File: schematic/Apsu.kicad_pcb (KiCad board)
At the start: 2 copper layers, 80 x 80 mm, 58 parts, among them J1 Conn_02x03_Odd_Even, J12 Conn_01x03, J13 Conn_01x02, J14 Conn_01x03_Female, J15 Conn_01x03, J16 Conn_01x03, J17 Conn_01x03, J18 Conn_01x02_Male, J19 Conn_01x02, J2 Conn_02x05_Odd_Even, J3 Conn_02x05_Odd_Even, J4 Conn_01x02, J5 Conn_01x02, J6 Conn_01x02, J7 Conn_01x02, J8 Conn_01x05, J9 Conn_01x08_Male, SW1 SW_DIP_x01, U1 ESP32-WROOM-32, U2 LM2595S-3.3, U3 PCA9685PW, U4 MAX11613, U5 MAX485E

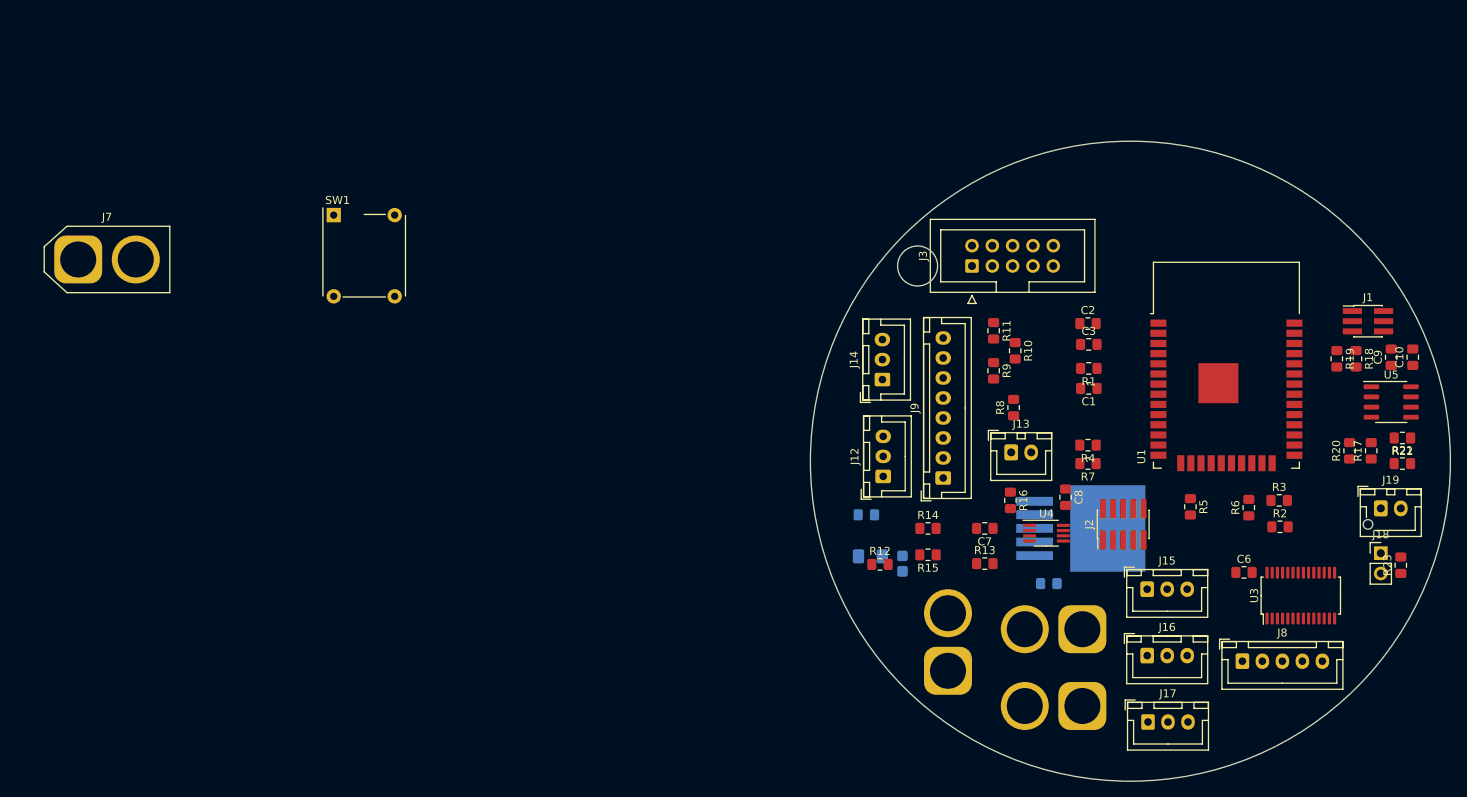
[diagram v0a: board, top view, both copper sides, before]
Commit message: new pcb design
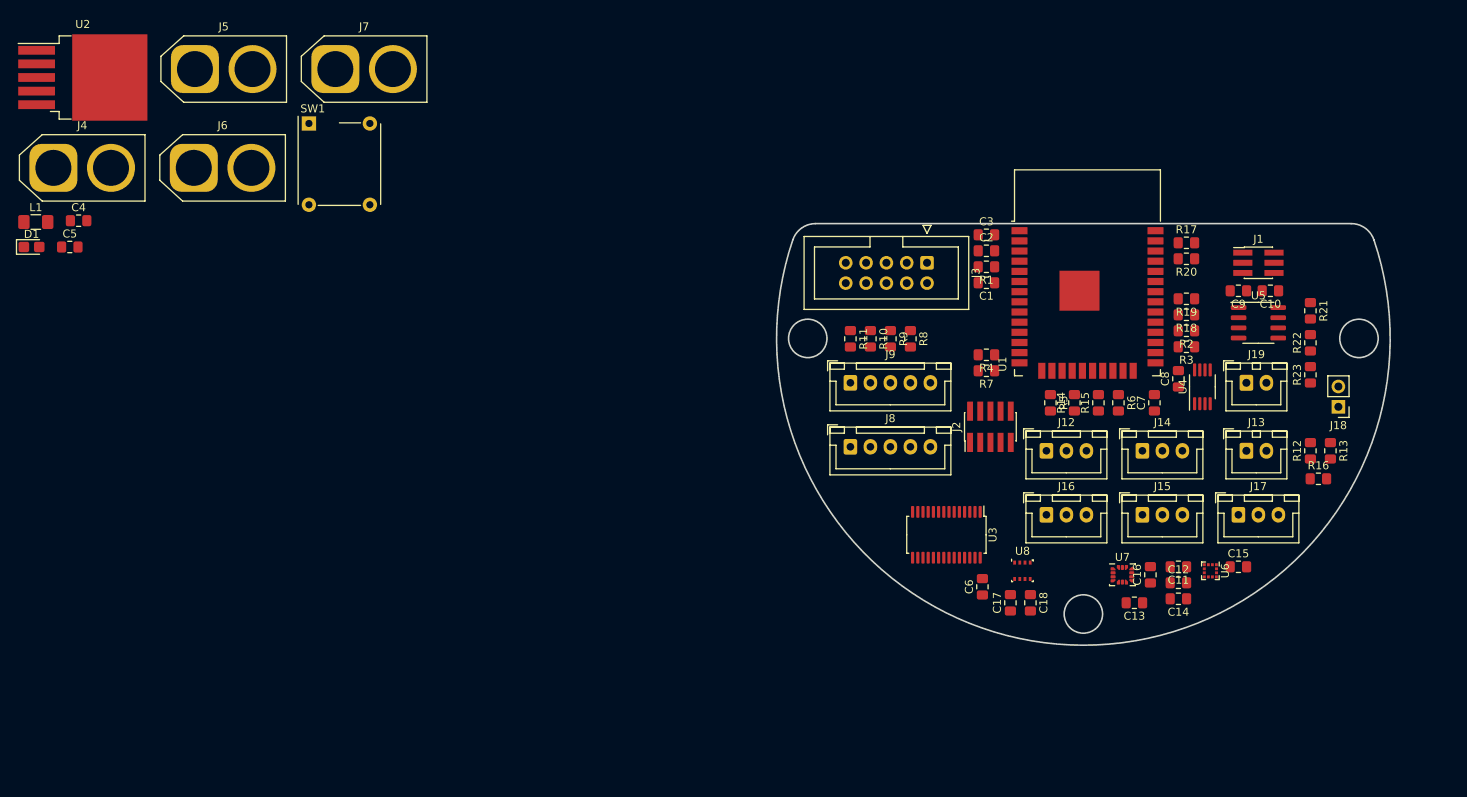
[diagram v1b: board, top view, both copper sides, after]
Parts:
- added C11: 220nF, Capacitor_SMD:C_0805_2012Metric_Pad1.15x1.40mm_HandSolder, F.Cu at (165.0, 123.0)
- added C12: 100nF, Capacitor_SMD:C_0805_2012Metric_Pad1.15x1.40mm_HandSolder, F.Cu at (165.0, 125.0)
- added C13: 100nF, Capacitor_SMD:C_0805_2012Metric_Pad1.15x1.40mm_HandSolder, F.Cu at (159.5, 127.5)
- added C14: 10uF, Capacitor_SMD:C_0805_2012Metric_Pad1.15x1.40mm_HandSolder, F.Cu at (165.0, 127.0)
- added C15: 100nF, Capacitor_SMD:C_0805_2012Metric_Pad1.15x1.40mm_HandSolder, F.Cu at (172.5, 123.0)
- added C16: 100nF, Capacitor_SMD:C_0805_2012Metric_Pad1.15x1.40mm_HandSolder, F.Cu at (161.5, 124.0)
- added C17: 100nF, Capacitor_SMD:C_0805_2012Metric_Pad1.15x1.40mm_HandSolder, F.Cu at (144.0, 127.5)
- added C18: 100nF, Capacitor_SMD:C_0805_2012Metric_Pad1.15x1.40mm_HandSolder, F.Cu at (146.5, 127.5)
- added U6: LIS2MDL, Package_LGA:LGA-12_2x2mm_P0.5mm, F.Cu at (169.0, 123.5)
- added U7: LSM6DSOX, Package_LGA:LGA-14_3x2.5mm_P0.5mm_LayoutBorder3x4y, F.Cu at (158.0, 124.0)
- added U8: BME280, Package_LGA:Bosch_LGA-8_2.5x2.5mm_P0.65mm_ClockwisePinNumbering, F.Cu at (145.5, 123.5)
- C4, C5, D1, J4, J5, J6, L1, U2: moved to F.Cu
- J19: footprint Connector_JST:JST_XH_B2B-XH-AM_1x02_P2.50mm_Vertical -> Connector_JST:JST_XH_B2B-XH-A_1x02_P2.50mm_Vertical
- J9: value Conn_01x08_Male -> Conn_01x05; footprint Connector_JST:JST_XH_B8B-XH-A_1x08_P2.50mm_Vertical -> Connector_JST:JST_XH_B5B-XH-A_1x05_P2.50mm_Vertical
- moved J4 145.2 mm to (24.4, 73.1), turned to 0 degrees
- moved U2 136.9 mm to (28.0, 61.8)
- moved J5 131.2 mm to (42.1, 60.8), turned to 0 degrees
- moved C4 129.5 mm to (27.5, 79.7)
- moved D1 115.8 mm to (21.6, 83.0), turned to 0 degrees
- moved J6 113.3 mm to (41.9, 73.1), turned to 0 degrees
- moved L1 112.4 mm to (22.2, 79.9), turned to 0 degrees
- moved C5 105.1 mm to (26.4, 83.0)
- moved J8 55.9 mm to (124.0, 108.0)
- moved R12 55.6 mm to (181.5, 108.5), turned to 90 degrees
- moved R13 45.4 mm to (184.0, 108.5), turned to 270 degrees
- moved U3 44.9 mm to (136.0, 119.0), turned to 270 degrees
- moved J7 40.0 mm to (59.6, 60.8)
- moved R16 38.6 mm to (182.5, 112.0), turned to 0 degrees
- moved R17 34.8 mm to (166.0, 82.5), turned to 0 degrees
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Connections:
- J9 pad 1: Net-(J9-Pad1) -> BLDC_right_z
- J9 pad 2: Net-(J9-Pad2) -> BLDC_M4
- J9 pad 3: GND -> BLDC_left_z
- J9 pad 4: Net-(J9-Pad4) -> BLDC_M3
- J9 pad 5: BLDC_M3 -> GND
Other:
- board size 80 x 80 mm -> 76.7 x 52.7 mm
